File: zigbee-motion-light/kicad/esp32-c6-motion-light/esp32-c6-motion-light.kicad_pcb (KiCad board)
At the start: 4 copper layers, 26.8 x 35 mm, 9 parts, among them Q1A1 2N7002, Q1B1 BSS84, U1 XIAO-ESP32-C6-DIP

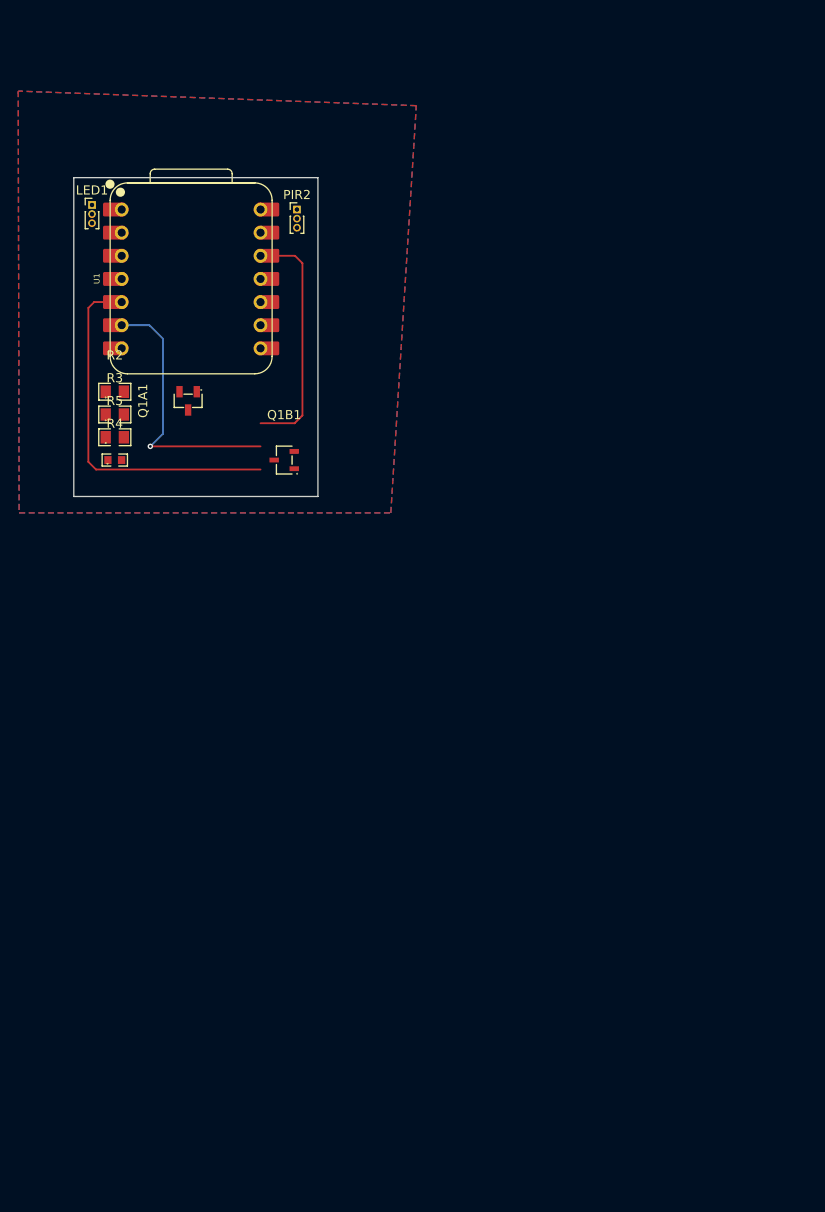
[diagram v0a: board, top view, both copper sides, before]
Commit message: feat: update kikad
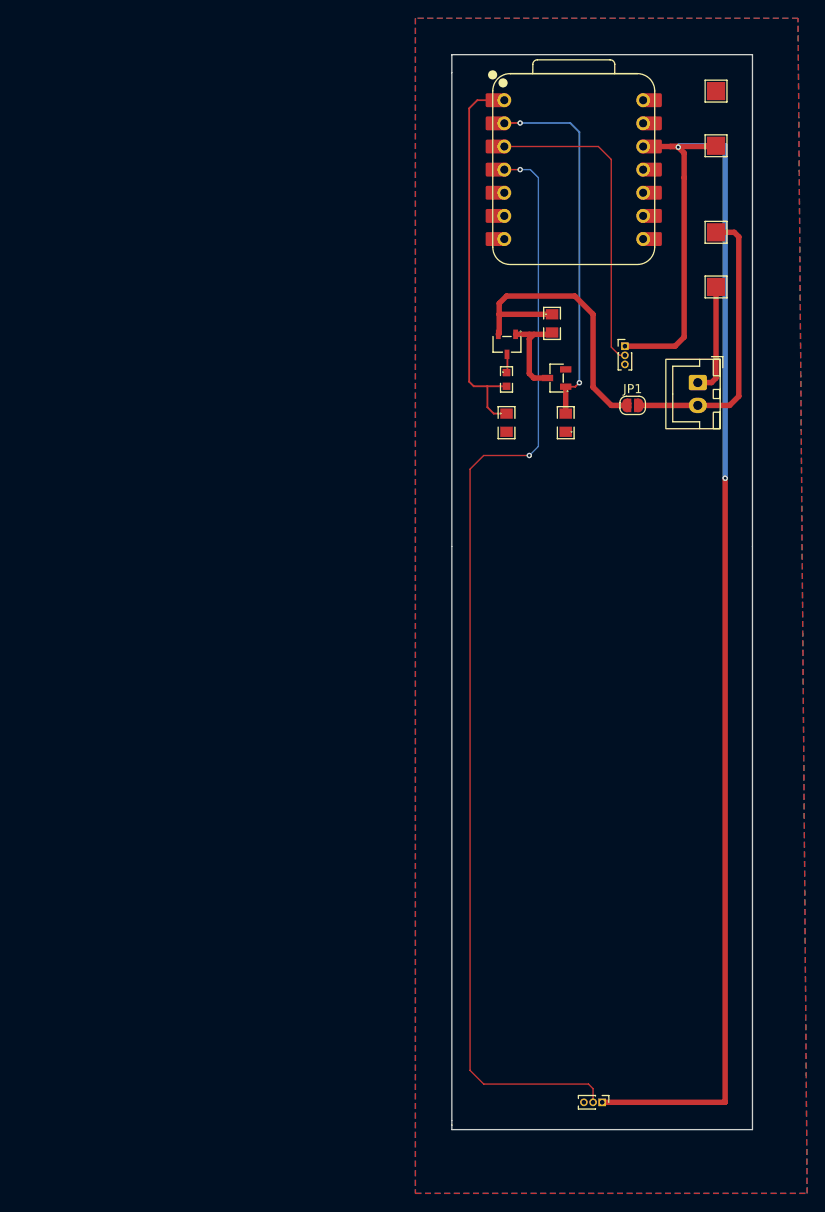
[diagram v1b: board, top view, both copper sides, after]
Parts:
- added J1: Conn_01x02, Connector_JST:JST_XH_B2B-XH-A_1x02_P2.50mm_Vertical, F.Cu at (127.0, 62.0)
- added JP1: Enabled for Batter Monitoring, Jumper:SolderJumper-2_P1.3mm_Open_RoundedPad1.0x1.5mm, F.Cu at (119.8, 64.5)
- added TP1: GND, TestPoint:TestPoint_Pad_2.0x2.0mm, F.Cu at (129.0, 30.0)
- added TP2: BATT+, TestPoint:TestPoint_Pad_2.0x2.0mm, F.Cu at (129.0, 45.5)
- added TP3: BATT-, TestPoint:TestPoint_Pad_2.0x2.0mm, F.Cu at (129.0, 51.5)
- added TP4: +3.3, TestPoint:TestPoint_Pad_2.0x2.0mm, F.Cu at (129.0, 36.0)
- moved LED1 113.3 mm to (116.5, 141.0), turned to -90 degrees
- moved R2 49.6 mm to (112.5, 66.4), turned to 90 degrees
- moved R3 49.0 mm to (111.0, 55.5), turned to -90 degrees
- moved R4 43.9 mm to (106.0, 61.6), turned to -90 degrees
- moved U1 43.7 mm to (113.4, 38.6)
- moved R5 43.0 mm to (106.0, 66.4), turned to -90 degrees
- moved Q1A1 40.5 mm to (111.5, 61.5), turned to 0 degrees
- moved PIR2 39.0 mm to (119.0, 58.0)
- moved Q1B1 27.6 mm to (106.0, 57.8), turned to 90 degrees
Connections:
- net +BATT renamed Net-(JP1-A)
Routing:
- net +3.3V: track 25.8 -> 159.7 mm, vias 0 -> 2
- net /LED_CONTROL: track 0.00 -> 124.0 mm, vias 0 -> 2
- net /BATTERY_MONITORING: track 0.00 -> 42.5 mm
- net /BATTERY_MONITORING_ENABLER: track 0.00 -> 41.3 mm, vias 0 -> 2
- net Net-(SCD41-SDA): track 39.2 -> 0.00 mm
- net /PIR_SENSOR: track 0.00 -> 34.8 mm
- net Net-(JP1-A): track 0.00 -> 33.2 mm
- net +BATT: track 0.00 -> 31.6 mm
- net unconnected-(U1-GPIO23/D5/SCL-Pad6): track 29.6 -> 0.00 mm, vias 1 -> 0
- net -BATT: track 0.00 -> 12.2 mm
- net Net-(Q1A1-D): track 0.00 -> 10.3 mm
- net Net-(Q1B1-D): track 0.00 -> 2.02 mm
- removed copper zone on In1.Cu, net GND
- removed copper zone on In2.Cu, net GND
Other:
- board size 26.8 x 35 mm -> 33 x 118 mm
